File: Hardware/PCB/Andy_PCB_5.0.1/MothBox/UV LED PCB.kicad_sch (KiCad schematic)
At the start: 24 parts, among them P4 External Attractor, Q10 BC817, Q7 BC817, Q8 BC817, Q9 BC817, U15 FDS4435BZ, U16 FDS4435BZ, U17 FDS4435BZ, U18 FDS4435BZ

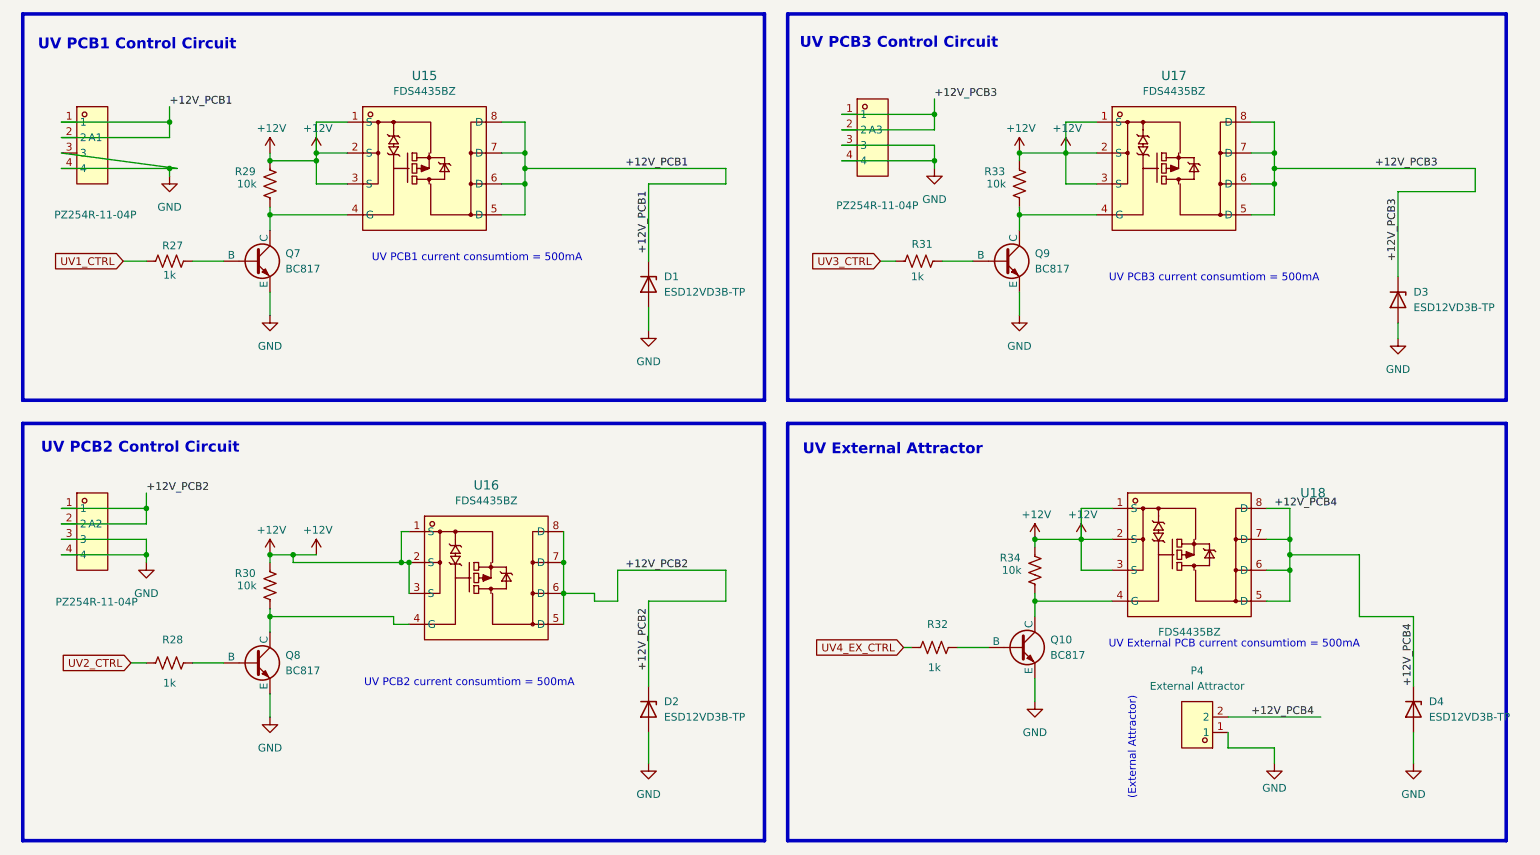
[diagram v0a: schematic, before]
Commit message: daily schematic updates
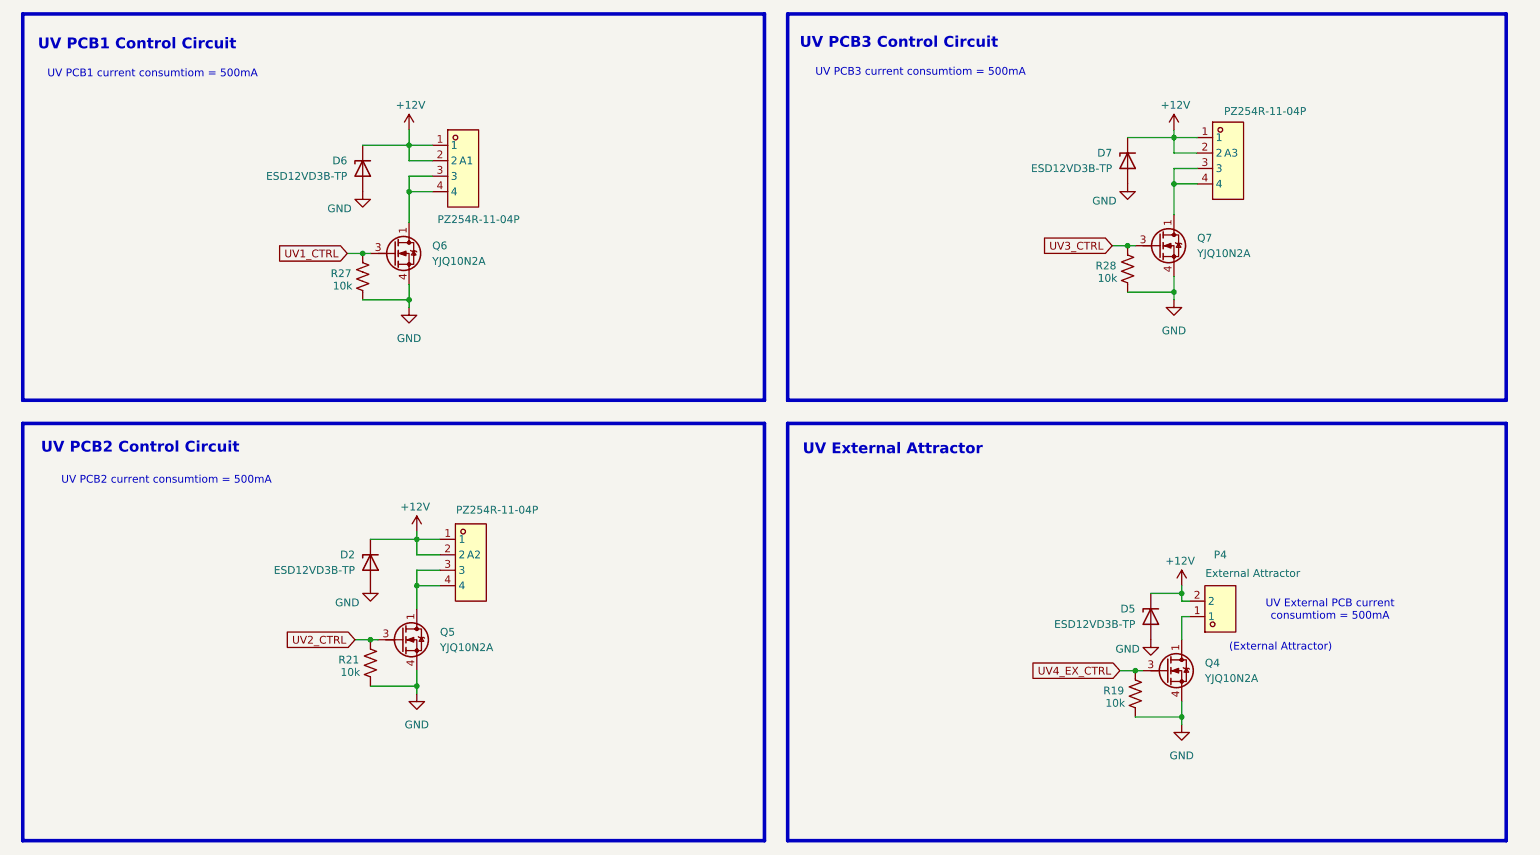
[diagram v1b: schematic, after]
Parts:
- removed D1, D3, D4: ESD12VD3B-TP, Diode_SMD:D_SOD-323, symbol MB_Library:ESD5Zxx
- removed Q10, Q7, Q8, Q9: BC817, Package_TO_SOT_SMD:SOT-23, symbol MB_Library:BC817_NPN_BJT
- removed R29, R30, R33, R34: 10k, Resistor_SMD:R_0805_2012Metric, symbol MB_Library:R_US
- removed R31, R32: 1k, Resistor_SMD:R_0805_2012Metric, symbol MB_Library:R_US
- removed U15, U16, U17, U18: FDS4435BZ, easyeda2kicad:SOIC-8_L5.0-W4.0-P1.27-LS6.0-BL, symbol MB_Library:FDS4435BZ
- added D5, D6, D7: ESD12VD3B-TP, Diode_SMD:D_SOD-323, symbol MB_Library:ESD5Zxx
- added Q4, Q5, Q6, Q7: YJQ10N2A, Pauls_Footprints:DFN2020-3, symbol _pauls_library:YJQ10N2A
- added R19, R21: 10k, Resistor_SMD:R_0805_2012Metric, symbol MB_Library:R_US
- R27, R28: value 1k -> 10k; LCSC Part no  C95781 -> C84376
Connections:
- net +12V_PCB1 is gone; now on net +12V: A1.1, A1.2
- net +12V_PCB2 is gone; now on net +12V: A2.1, A2.2, D2.1 (K)
- net +12V_PCB3 is gone; now on net +12V: A3.1, A3.2
- net +12V_PCB4 is gone; now on net +12V: P4.2
- net +12V: now also D5.1 (K), D6.1 (K), D7.1 (K)
- net GND: now also R27.1, R28.1, D5.2 (A), D6.2 (A), D7.2 (A), Q4.4 (S), Q4.7 (S), Q5.4 (S), Q5.7 (S), Q6.4 (S), Q6.7 (S), Q7.4 (S), Q7.7 (S), R19.1, R21.1; no longer A1.3, A1.4, A2.3, A2.4, A3.3, A3.4, P4.1
- net UV1_CTRL: now also Q6.3 (D)
- net UV2_CTRL: now also Q5.3 (D), R21.2; no longer R28.2
- net UV3_CTRL: now also R28.2, Q7.3 (D)
- net UV4_EX_CTRL: now also Q4.3 (D), R19.2
- new net: P4.1, Q4.1 (D), Q4.2 (D), Q4.3 (D), Q4.5 (D), Q4.6 (D), Q4.8 (D)
- new net: A1.3, A1.4, Q6.1 (D), Q6.2 (D), Q6.3 (D), Q6.5 (D), Q6.6 (D), Q6.8 (D)
- new net: A2.3, A2.4, Q5.1 (D), Q5.2 (D), Q5.3 (D), Q5.5 (D), Q5.6 (D), Q5.8 (D)
- new net: A3.3, A3.4, Q7.1 (D), Q7.2 (D), Q7.3 (D), Q7.5 (D), Q7.6 (D), Q7.8 (D)
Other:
- moved on the sheet: A1, A2, A3, D2, P4
